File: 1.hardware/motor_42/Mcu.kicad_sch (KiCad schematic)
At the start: 26 parts, among them U2 STM32F103CBTx, Y1 YSX321SL_12Mhz

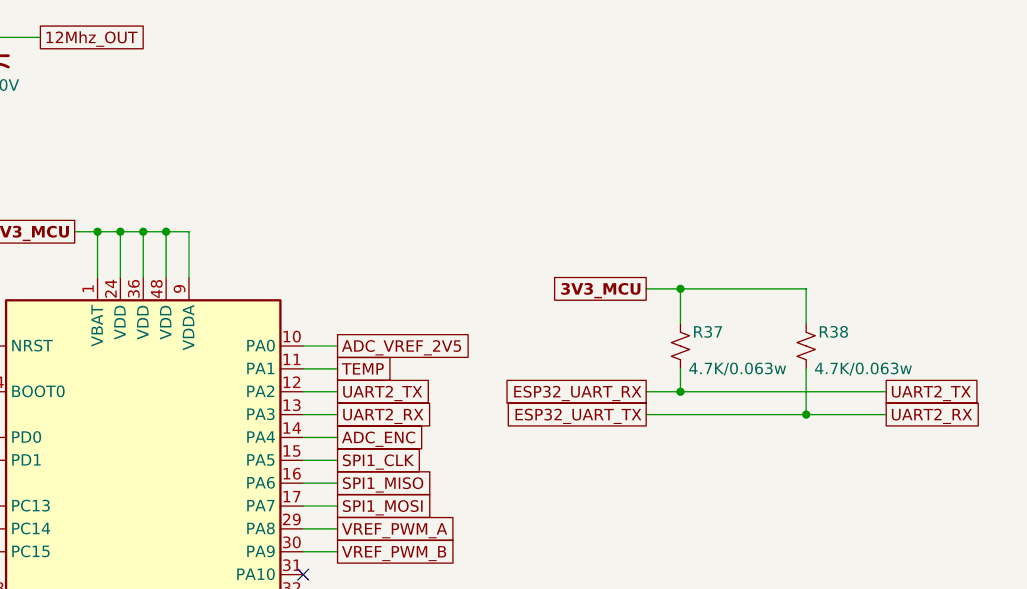
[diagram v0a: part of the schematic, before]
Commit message: 중간 저장
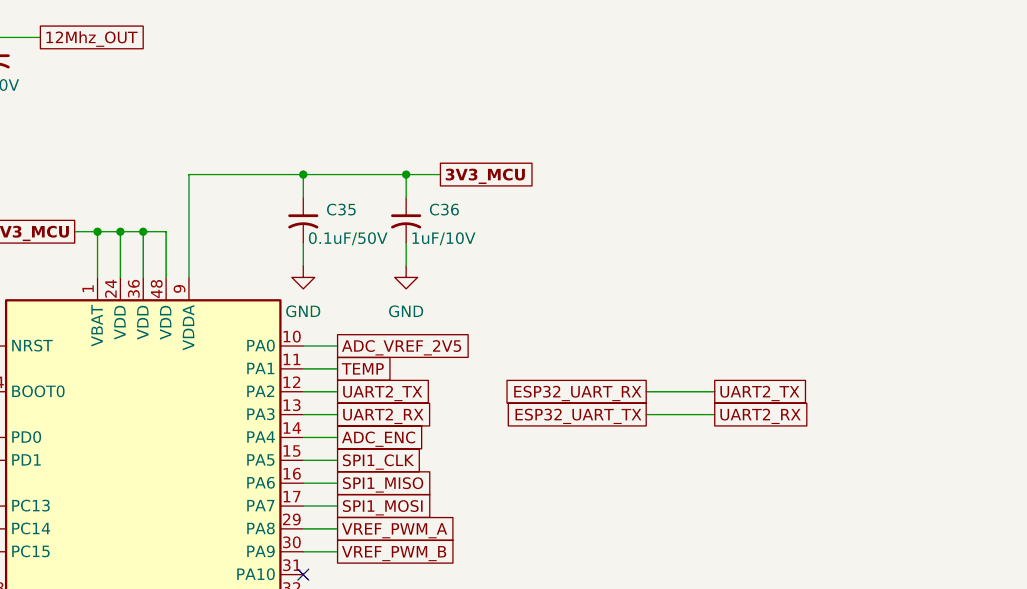
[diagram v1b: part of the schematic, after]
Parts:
- removed R37, R38: 4.7K/0.063w, Resistor_SMD:R_0402_1005Metric, symbol Device:R_Small_US
- added C35: 0.1uF/50V, Capacitor_SMD:C_0402_1005Metric, symbol Device:C_Small_US
- added C36: 1uF/10V, Capacitor_SMD:C_0402_1005Metric, symbol Device:C_Small_US
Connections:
- net 3V3: now also C35.1, C36.1
- net GND: now also C35.2, C36.2
